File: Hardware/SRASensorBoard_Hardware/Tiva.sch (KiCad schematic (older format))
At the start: 8 parts

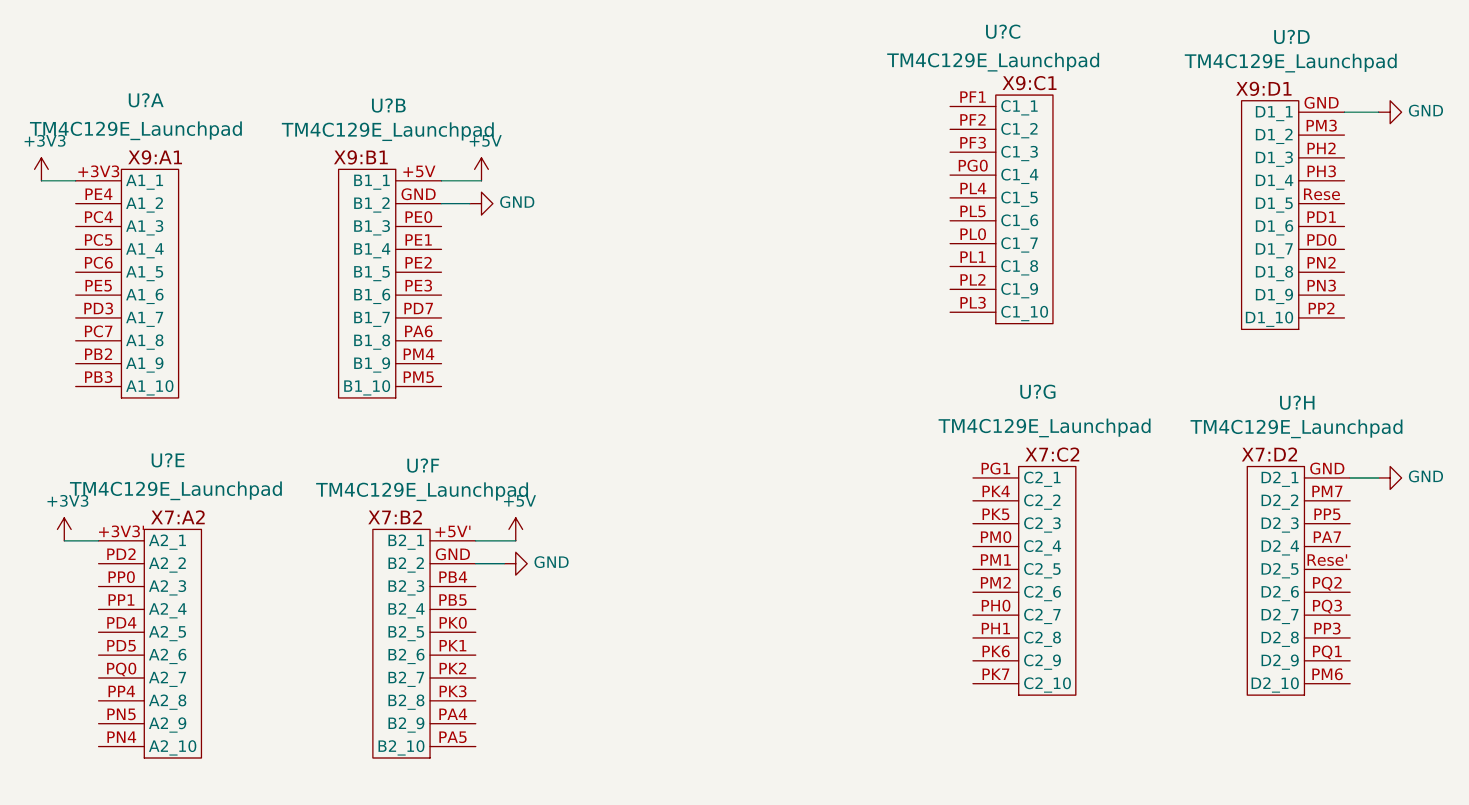
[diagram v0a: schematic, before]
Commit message: Added Okis to board
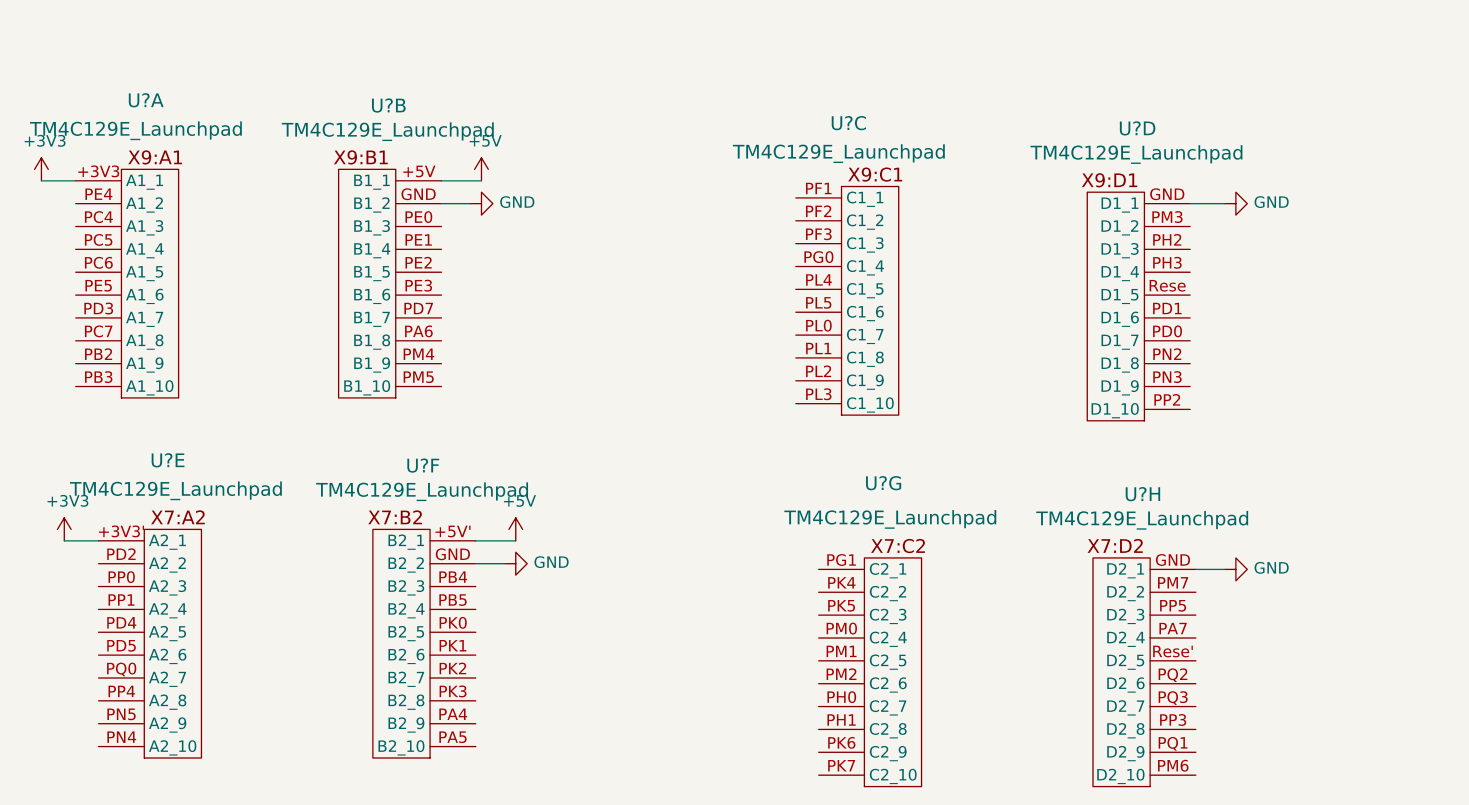
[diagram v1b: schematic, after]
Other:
- moved on the sheet: U?C, U?D, U?G, U?H
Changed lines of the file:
@@
 L MRDT_Shields:TM4C129E_Launchpad U?
 U 3 1 614D9ED3
-P 6100 2150
-F 0 "U?" H 6050 3425 60  0000 L CNN
-F 1 "TM4C129E_Launchpad" H 5625 3300 60  0000 L CNN
-F 2 "" H 6100 2150 60  0001 C CNN
-F 3 "" H 6100 2150 60  0001 C CNN
-	3    6100 2150
+P 5425 2550
+F 0 "U?" H 5375 3825 60  0000 L CNN
+F 1 "TM4C129E_Launchpad" H 4950 3700 60  0000 L CNN
+F 2 "" H 5425 2550 60  0001 C CNN
+F 3 "" H 5425 2550 60  0001 C CNN
+	3    5425 2550
 	1    0    0    -1
 $EndComp
@@
 L MRDT_Shields:TM4C129E_Launchpad U?
 U 4 1 614DBFEF
-P 7425 2175
-F 0 "U?" H 7456 3452 60  0000 C CNN
-F 1 "TM4C129E_Launchpad" H 7456 3346 60  0000 C CNN
-F 2 "" H 7425 2175 60  0001 C CNN
-F 3 "" H 7425 2175 60  0001 C CNN
-	4    7425 2175
+P 6750 2575
+F 0 "U?" H 6781 3852 60  0000 C CNN
+F 1 "TM4C129E_Launchpad" H 6781 3746 60  0000 C CNN
+F 2 "" H 6750 2575 60  0001 C CNN
+F 3 "" H 6750 2575 60  0001 C CNN
+	4    6750 2575
 	-1   0    0    -1
 $EndComp
@@
 L MRDT_Shields:TM4C129E_Launchpad U?
 U 7 1 614E25CE
-P 6200 3775
-F 0 "U?" H 6200 5100 60  0000 L CNN
-F 1 "TM4C129E_Launchpad" H 5850 4950 60  0000 L CNN
-F 2 "" H 6200 3775 60  0001 C CNN
-F 3 "" H 6200 3775 60  0001 C CNN
-	7    6200 3775
+P 5525 4175
+F 0 "U?" H 5525 5500 60  0000 L CNN
+F 1 "TM4C129E_Launchpad" H 5175 5350 60  0000 L CNN
+F 2 "" H 5525 4175 60  0001 C CNN
+F 3 "" H 5525 4175 60  0001 C CNN
+	7    5525 4175
 	1    0    0    -1
 $EndComp
@@
 L MRDT_Shields:TM4C129E_Launchpad U?
 U 8 1 614E511C
-P 7450 3775
-F 0 "U?" H 7481 5052 60  0000 C CNN
-F 1 "TM4C129E_Launchpad" H 7481 4946 60  0000 C CNN
-F 2 "" H 7450 3775 60  0001 C CNN
-F 3 "" H 7450 3775 60  0001 C CNN
-	8    7450 3775
+P 6775 4175
+F 0 "U?" H 6806 5452 60  0000 C CNN
+F 1 "TM4C129E_Launchpad" H 6806 5346 60  0000 C CNN
+F 2 "" H 6775 4175 60  0001 C CNN
+F 3 "" H 6775 4175 60  0001 C CNN
+	8    6775 4175
 	-1   0    0    -1
 $EndComp
@@
 L power:GND #PWR?
 U 1 1 614FF513
-P 7775 2825
-F 0 "#PWR?" H 7775 2575 50  0001 C CNN
-F 1 "GND" V 7780 2697 50  0000 R CNN
-F 2 "" H 7775 2825 50  0001 C CNN
-F 3 "" H 7775 2825 50  0001 C CNN
-	1    7775 2825
+P 7100 3225
+F 0 "#PWR?" H 7100 2975 50  0001 C CNN
+F 1 "GND" V 7105 3097 50  0000 R CNN
+F 2 "" H 7100 3225 50  0001 C CNN
+F 3 "" H 7100 3225 50  0001 C CNN
+	1    7100 3225
 	0    -1   -1   0
 $EndComp
@@
 L power:GND #PWR?
 U 1 1 61500297
-P 7775 1225
-F 0 "#PWR?" H 7775 975 50  0001 C CNN
-F 1 "GND" V 7780 1097 50  0000 R CNN
-F 2 "" H 7775 1225 50  0001 C CNN
-F 3 "" H 7775 1225 50  0001 C CNN
-	1    7775 1225
+P 7100 1625
+F 0 "#PWR?" H 7100 1375 50  0001 C CNN
+F 1 "GND" V 7105 1497 50  0000 R CNN
+F 2 "" H 7100 1625 50  0001 C CNN
+F 3 "" H 7100 1625 50  0001 C CNN
+	1    7100 1625
 	0    -1   -1   0
 $EndComp
@@
 $EndComp
 Wire Wire Line
-	7625 1225 7775 1225
+	6950 1625 7100 1625
 Wire Wire Line
-	7650 2825 7775 2825
+	6975 3225 7100 3225
 Wire Wire Line
 	3825 3200 3950 3200
